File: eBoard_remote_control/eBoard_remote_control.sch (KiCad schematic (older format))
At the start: 42 parts, among them J1 SWDIO_conn, P1 USB, U1 MDBT42, U2 AP2112(3.3V), U3 MCP73831T-2ACI/OT, U4 CP2104, U5 AH49ENTR-G1, U6 AH49ENTR-G1, U7 AH49ENTR-G1, X2 JSTPH, X4 32.768

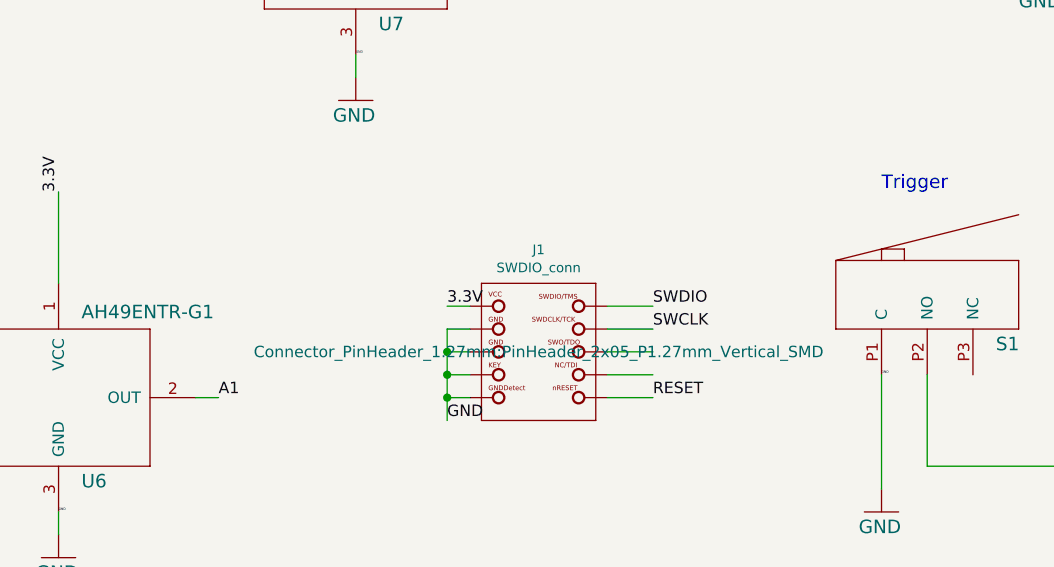
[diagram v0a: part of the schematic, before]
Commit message: V2.1
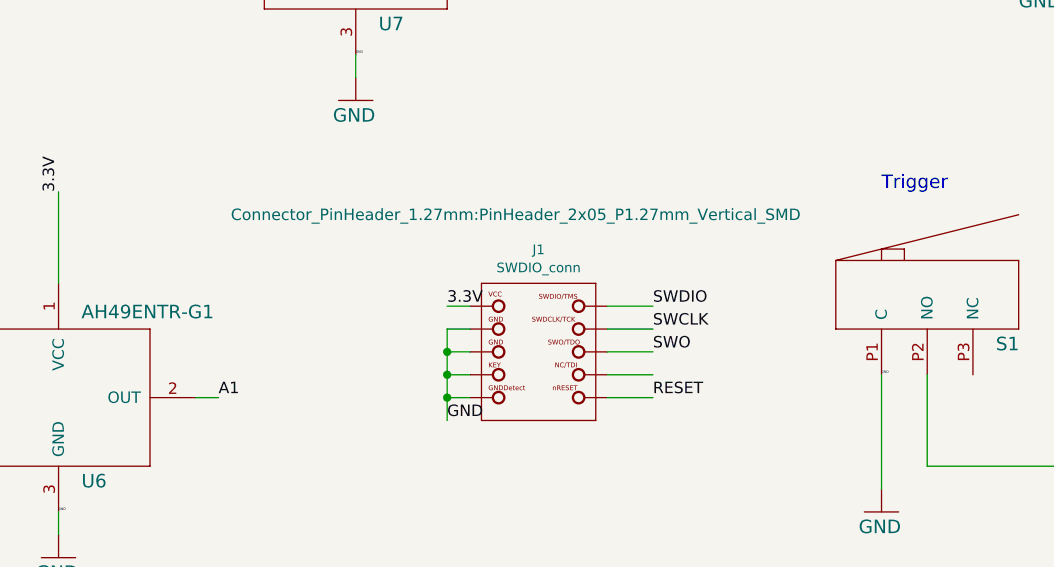
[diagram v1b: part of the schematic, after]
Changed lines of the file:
@@
 F 0 "J1" H 11700 4547 42  0000 C CNN
 F 1 "SWDIO_conn" H 11700 4468 42  0000 C CNN
-F 2 "Connector_PinHeader_1.27mm:PinHeader_2x05_P1.27mm_Vertical_SMD" H 11700 4100 50  0000 C CNN
+F 2 "Connector_PinHeader_1.27mm:PinHeader_2x05_P1.27mm_Vertical_SMD" H 11600 4700 50  0000 C CNN
 F 3 "" H 11700 4100 50  0001 C CNN
 	1    11700 4100
@@
 Wire Wire Line
 	11300 3900 11400 3900
+Text Label 12200 4100 0    50   ~ 0
+SWO
 $EndSCHEMATC

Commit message: this
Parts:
- removed DIS1: OLED, eBoard_remote_control:OLED, symbol eBoard_remote_control-eagle-import:OLED
- added U8: SSD1306, eBoard_remote_control:SSD1306_OLED-0.91-128x32, symbol SSD1306_OLED-0.91-128x32:SSD1306
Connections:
- wire segments 188 -> 183
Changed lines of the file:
@@
-GND
-Wire Wire Line
-	14000 2000 13900 2000
-Wire Wire Line
-	13900 2000 13900 2400
-Text Label 14000 2000 0    10   ~ 0
 GND
 Wire Wire Line
@@
 Text Label 14100 3800 1    50   ~ 0
 3.3V
-Text Label 12300 1900 2    50   ~ 0
-3.3V
 Wire Wire Line
 	3100 7300 3000 7300
 Text Label 3000 7300 2    50   ~ 0
 SDA
-Text Label 12300 1700 2    50   ~ 0
-SDA
 Wire Wire Line
 	3100 7400 3000 7400
 Text Label 3000 7400 2    50   ~ 0
-SCL
-Text Label 12300 1800 2    50   ~ 0
 SCL
 Wire Wire Line
@@
 	1    15400 4300
 	0    1    1    0
-$EndComp
-$Comp
-L eBoard_remote_control-eagle-import:OLED DIS1
-U 1 0 E925ABD7
-P 14900 1900
-F 0 "DIS1" H 14900 1650 59  0000 C CNN
-F 1 "OLED" H 15070 2000 59  0000 C CNN
-F 2 "eBoard_remote_control:OLED" H 14900 1900 50  0001 C CNN
-F 3 "" H 14900 1900 50  0001 C CNN
-	1    14900 1900
-	1    0    0    -1
-$EndComp
-$Comp
-L eBoard_remote_control-eagle-import:GND #GND04
-U 1 0 12C122FD
-P 13900 2500
-F 0 "#GND04" H 13900 2500 50  0001 C CNN
-F 1 "GND" H 13800 2400 59  0000 L BNN
-F 2 "" H 13900 2500 50  0001 C CNN
-F 3 "" H 13900 2500 50  0001 C CNN
-	1    13900 2500
-	1    0    0    -1
 $EndComp
 $Comp
@@
 Wire Wire Line
 	9600 3400 9600 3800
-Wire Wire Line
-	12300 1800 14000 1800
-Wire Wire Line
-	12300 1700 14000 1700
-Wire Wire Line
-	12300 1900 14000 1900
 $Comp
 L eBoard_remote_control-eagle-import:CAP_CERAMIC0603_NO C9
@@
 Text Label 12200 4100 0    50   ~ 0
 SWO
+$Comp
+L SSD1306_OLED-0.91-128x32:SSD1306 U8
+U 1 1 5CC03FF3
+P 13900 2350
+F 0 "U8" H 13900 3187 60  0000 C CNN
+F 1 "SSD1306" H 13900 3081 60  0000 C CNN
+F 2 "eBoard_remote_control:SSD1306_OLED-0.91-128x32" H 13900 2350 60  0001 C CNN
+F 3 "" H 13900 2350 60  0001 C CNN
+	1    13900 2350
+	1    0    0    -1
+$EndComp
 $EndSCHEMATC
